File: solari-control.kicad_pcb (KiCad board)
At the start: 2 copper layers, 80 x 80 mm, 108 parts, among them J1 Conn_01x04, J2 A5081WV-5P, J3 A5081WR-5P, J4 AVR-ISP-6, J5 DIL8, J6 Conn_01x04, Q1 AO3401A, Q10 AO3400A, Q11 AO3401A, Q12 AO3400A, Q2 AO3400A, Q3 AO3401A, Q4 AO3400A, Q5 AO3401A, Q6 AO3401A, Q7 AO3401A, Q8 AO3401A, Q9 AO3401A, U1 VO0631T, U10 PC817, U11 PC817, U2 L78L05_SOT89, U3 VO0631T, U4 PC817, U5 PC817, U6 VO0631T, U7 ATmega328P-A, U8 VO0631T, U9 VO0631T, Y1 14.7456 MHz

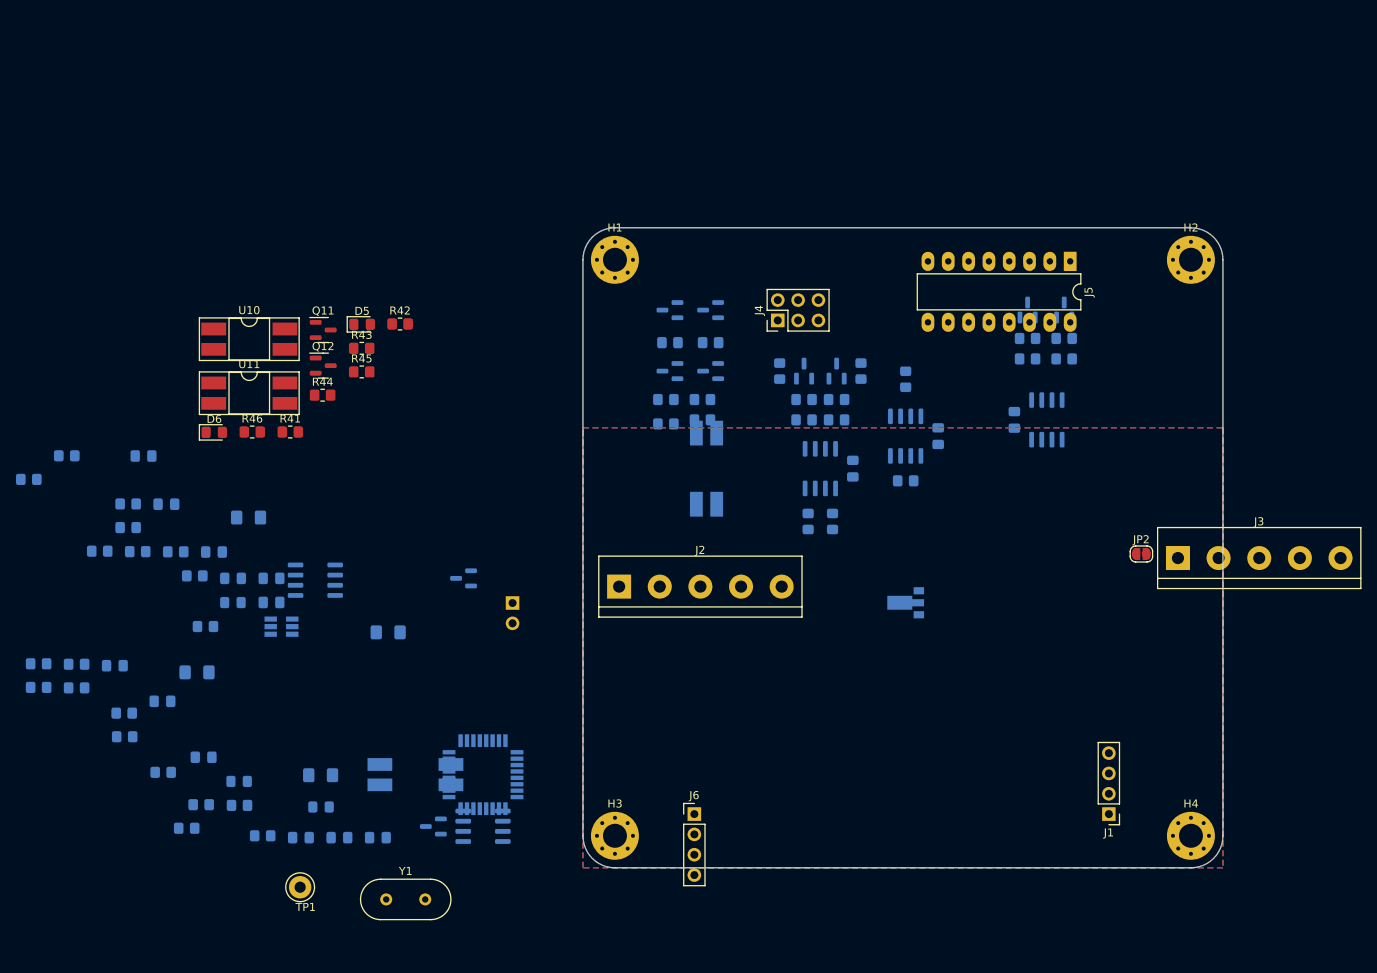
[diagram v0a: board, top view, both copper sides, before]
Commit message: PCB: place parts into chunks.
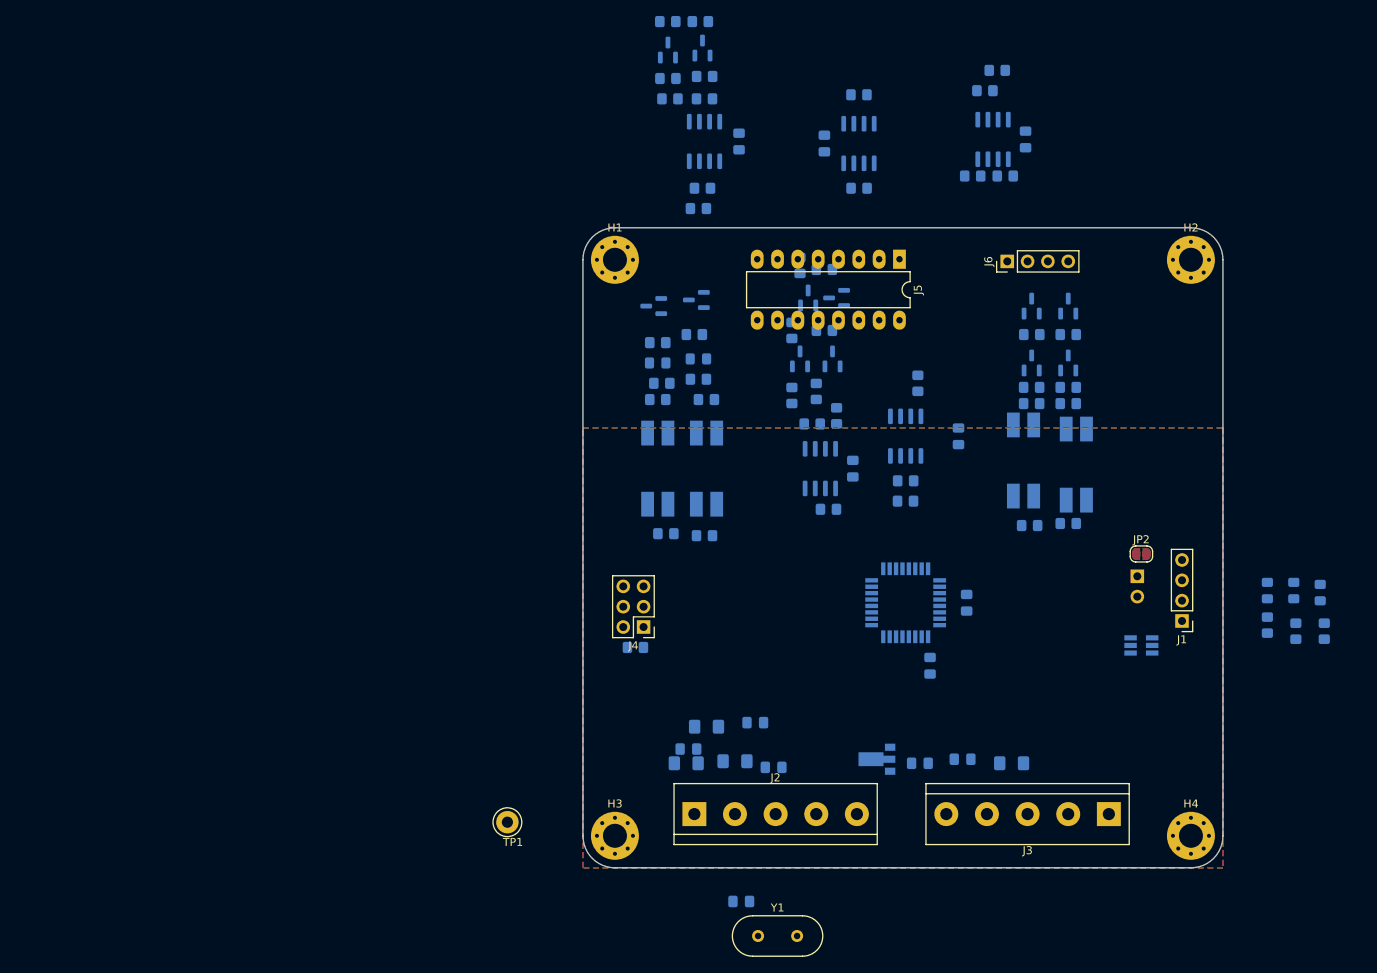
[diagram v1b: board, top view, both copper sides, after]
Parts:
- removed C14: 22u/25V, Capacitor_SMD:C_0805_2012Metric_Pad1.18x1.45mm_HandSolder
- removed C15: 100n, Capacitor_SMD:C_0805_2012Metric_Pad1.18x1.45mm_HandSolder
- D5, D6, Q11, Q12, R41, R42, R43, R44, R45, R46, U10, U11: moved to B.Cu
- moved R27 152.6 mm to (229.1, 90.4), turned to -90 degrees
- moved R28 146.2 mm to (232.7, 90.4), turned to -90 degrees
- moved D6 139.7 mm to (232.2, 85.6), turned to -90 degrees
- moved D4 129.3 mm to (225.6, 85.3), turned to -90 degrees
- moved R29 126.5 mm to (174.5, 23.4)
- moved R22 123.5 mm to (190.2, 22.9)
- moved D5 121.1 mm to (228.9, 85.3), turned to -90 degrees
- moved R23 118.2 mm to (192.8, 33.5)
- moved C9 117.1 mm to (195.3, 29.0), turned to -90 degrees
- moved R31 111.4 mm to (150.6, 21.3)
- moved R1 110.8 mm to (180.3, 71.6)
- moved R34 109.9 mm to (155.2, 21.1)
- moved R25 109.3 mm to (188.7, 33.5)
- moved D1 107.5 mm to (209.8, 92.2)
- moved R33 105.9 mm to (150.9, 23.9)
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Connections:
- R42 pad 1: VDO -> Net-(Q11-Pad1)
- R42 pad 2: Net-(Q11-Pad1) -> VDO
